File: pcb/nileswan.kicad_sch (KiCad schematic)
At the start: 8 parts, among them J1 Micro_SD_Card_Det_Hirose_DM3AT

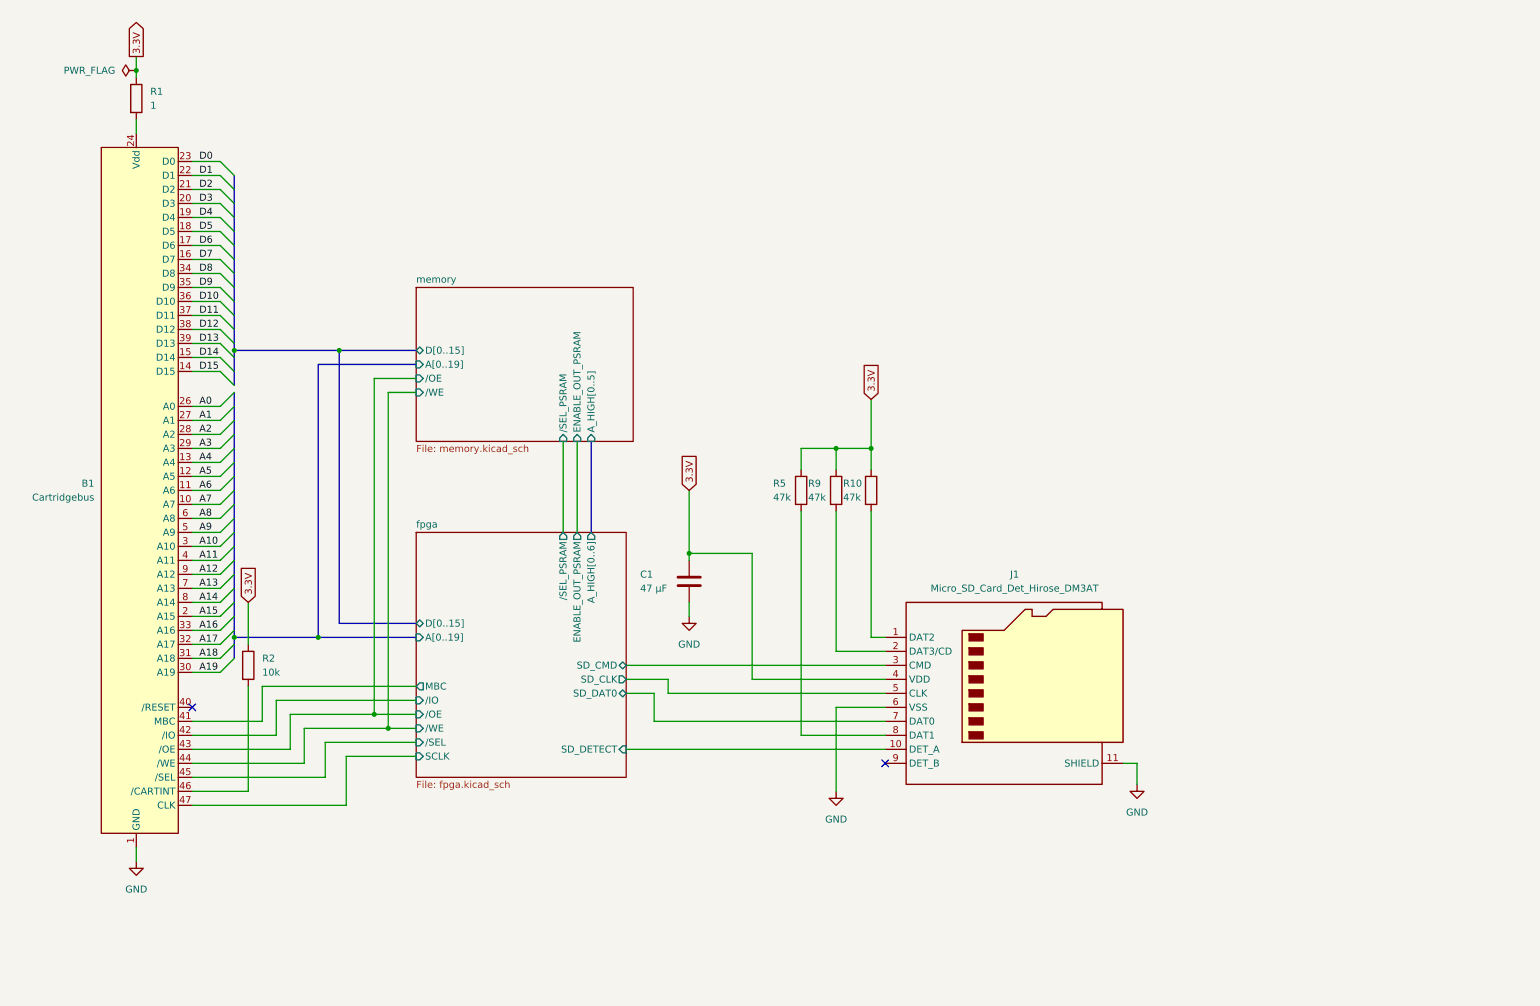
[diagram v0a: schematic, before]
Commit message: second pcb iteration
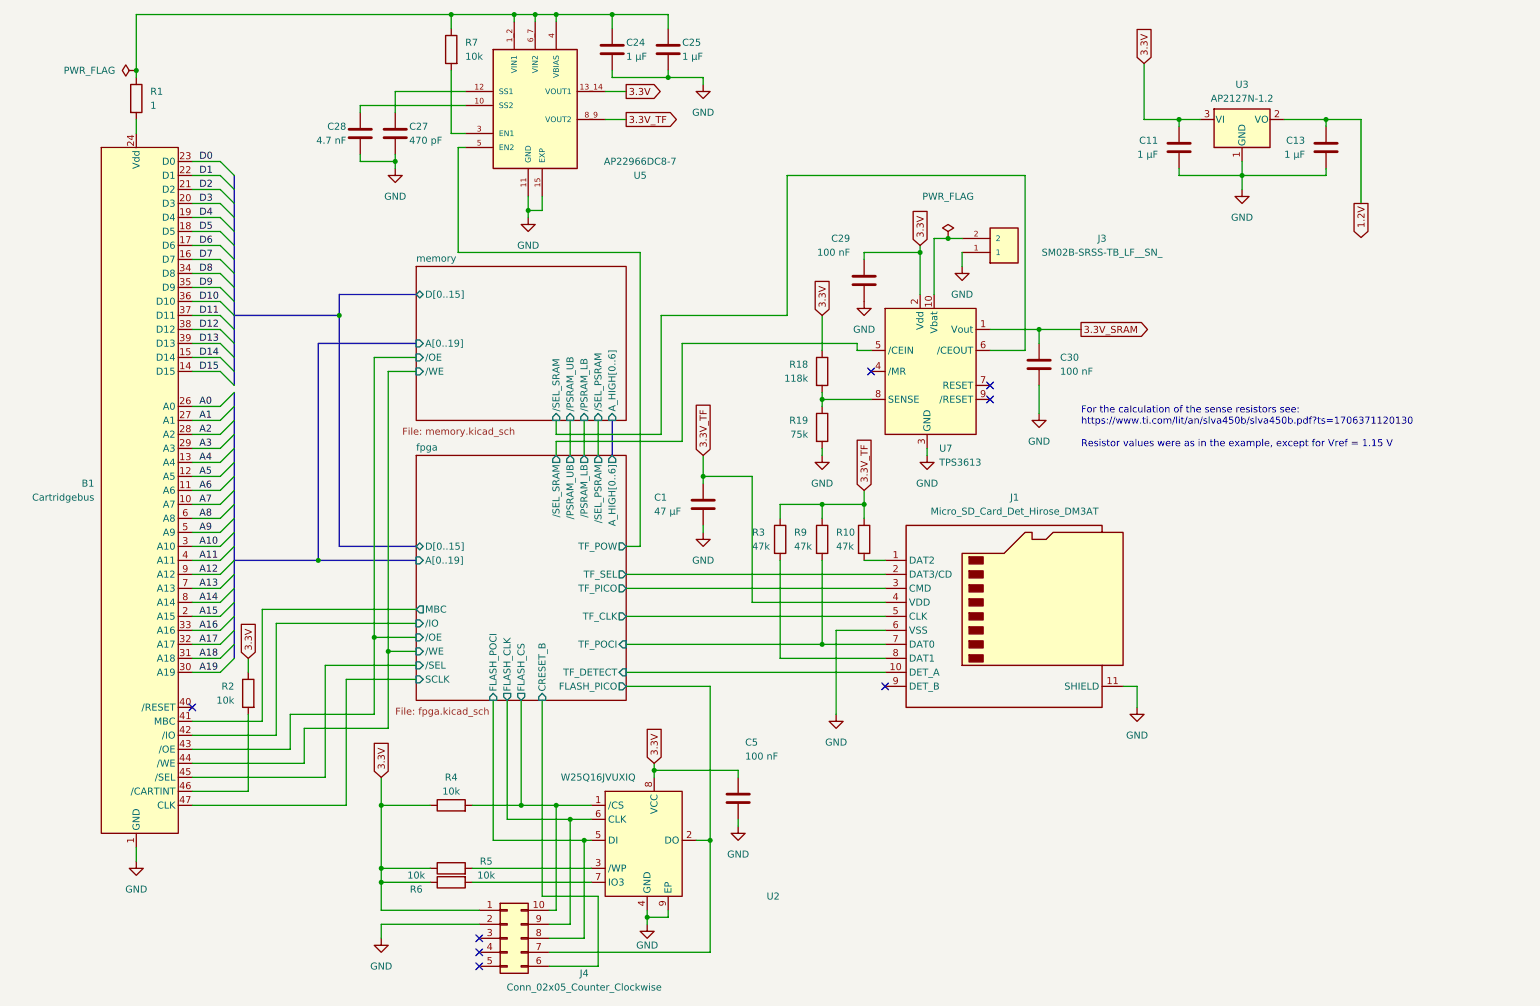
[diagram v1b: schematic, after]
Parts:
- added C11, C13, C24, C25: 1 μF, Capacitor_SMD:C_0603_1608Metric, symbol Device:C
- added C27: 470 pF, Capacitor_SMD:C_0402_1005Metric, symbol Device:C
- added C28: 4.7 nF, Capacitor_SMD:C_0402_1005Metric, symbol Device:C
- added C29, C30, C5: 100 nF, Capacitor_SMD:C_0402_1005Metric, symbol Device:C
- added J3: SM02B-SRSS-TB_LF__SN_, snapeda:SM02B-SRSS-TB_LF__SN_, symbol SM02B-SRSS-TB:SM02B-SRSS-TB_LF__SN_
- added J4: Conn_02x05_Counter_Clockwise, Connector:Tag-Connect_TC2050-IDC-NL_2x05_P1.27mm_Vertical, symbol Connector_Generic:Conn_02x05_Counter_Clockwise
- added R18: 118k, Resistor_SMD:R_0402_1005Metric, symbol Device:R
- added R19: 75k, Resistor_SMD:R_0402_1005Metric, symbol Device:R
- added R3: 47k, Resistor_SMD:R_0402_1005Metric, symbol Device:R
- added R4, R6, R7: 10k, Resistor_SMD:R_0402_1005Metric, symbol Device:R
- added U2: W25Q16JVUXIQ, snapeda:SON50P300X200X60-9N, symbol nileswan:W25Q16JVUXIQ
- added U3: AP2127N-1.2, Package_TO_SOT_SMD:SOT-23, symbol Regulator_Linear:AP2127N-1.2
- added U5: AP22966DC8-7, snapeda:IC_AP22966DC8-7, symbol AP22966DC8-7:AP22966DC8-7
- added U7: TPS3613, Package_SO:VSSOP-10_3x3mm_P0.5mm, symbol nileswan:TPS3613
- R10, R2, R9: footprint Resistor_SMD:R_0603_1608Metric -> Resistor_SMD:R_0402_1005Metric
- R5: value 47k -> 10k; footprint Resistor_SMD:R_0603_1608Metric -> Resistor_SMD:R_0402_1005Metric
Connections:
- net fpga/SD_DAT0 is gone; now on net fpga/TF_POCI: J1.7 (DAT0)
- net 3.3V: now also C11.1, C29.1, C5.1, J4.1 (Pin_1), R18.1, R4.1, R6.1, U2.8 (VCC), U3.3 (VI), U5.13_14 (VOUT1), U7.2 (Vdd); no longer C1.1, J1.4 (VDD), R1.1, R10.1, R9.1
- net GND: now also C11.2, C13.2, C24.2, C25.2, C27.2, C28.2, C29.2, C30.2, C5.2, J3.1, J4.2 (Pin_2), R19.2, U2.4 (GND), U2.9 (EP), U3.1 (GND), U5.11 (GND), U5.15 (EXP), U7.3 (GND)
- net at J1.8 (DAT1): now also R3.2; no longer R5.2
- net fpga/TF_POCI: now reaches R9.2
- net fpga/TF_POCI: no longer J1.2 (DAT3/CD)
- net fpga/SD_CLK renamed fpga/TF_CLK
- net fpga/SD_CMD renamed fpga/TF_PICO
- net fpga/SD_DETECT renamed fpga/TF_DETECT
- new net: J3.2, U7.10 (Vbat)
- new net: R18.2, R19.1, U7.8 (SENSE)
- new net: C24.1, C25.1, R1.1, R7.1, U5.1_2 (VIN1), U5.4 (VBIAS), U5.6_7 (VIN2)
- new net: C28.1, U5.10 (SS2)
- new net: C27.1, U5.12 (SS1)
- new net: R7.2, U5.3 (EN1)
- new net: R5.2, U2.3 (/WP)
- new net: R6.2, U2.7 (IO3)
- new net 1.2V: C13.1, U3.2 (VO)
- new net 3.3V_SRAM: C30.1, U7.1 (Vout)
- new net 3.3V_TF: C1.1, J1.4 (VDD), R10.1, R3.1, R9.1, U5.8_9 (VOUT2)
- new net fpga/CRESET_B: J4.6 (Pin_6)
- new net fpga/FLASH_CLK: J4.9 (Pin_9), U2.6 (CLK)
- new net fpga/FLASH_CS: J4.10 (Pin_10), R4.2, U2.1 (/CS)
- new net fpga/FLASH_PICO: J4.7 (Pin_7), U2.2 (DO)
- new net fpga/FLASH_POCI: J4.8 (Pin_8), U2.5 (DI)
- new net fpga/TF_POW: U5.5 (EN2)
- new net fpga/TF_SEL: J1.2 (DAT3/CD)
- new net fpga//SEL_SRAM: U7.5 (/CEIN)
- new net memory//SEL_SRAM: U7.6 (/CEOUT)
- no-connect marks 2 -> 8
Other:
- sheet fpga ports: added CRESET_B, FLASH_CLK, FLASH_CS, FLASH_PICO, FLASH_POCI, TF_CLK, TF_DETECT, TF_PICO, TF_POCI, TF_POW, TF_SEL, /PSRAM_LB, /PSRAM_UB, /SEL_SRAM; removed ENABLE_OUT_PSRAM, SD_CLK, SD_CMD, SD_DAT0, SD_DETECT
- sheet memory ports: added A_HIGH[0..6], /PSRAM_LB, /PSRAM_UB, /SEL_SRAM; removed A_HIGH[0..5], ENABLE_OUT_PSRAM
- note added: "For the calculation of the sense resistors see: https://www.ti.com/lit/an/slva450b/slva450b.pdf?ts=1706371120130 Resistor values were as in the example, except for Vref = 1.15 V"
- moved on the sheet: C1, J1, R10, R2, R9
